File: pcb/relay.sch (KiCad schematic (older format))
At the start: 22 parts, among them IC1 ATTINY13-P, P1 CONN_01X02, P2 CONN_02X20, Q1 BC548, Q2 BC548, SW1 SW_PUSH, U1 78L05, U2 DX_MODULE

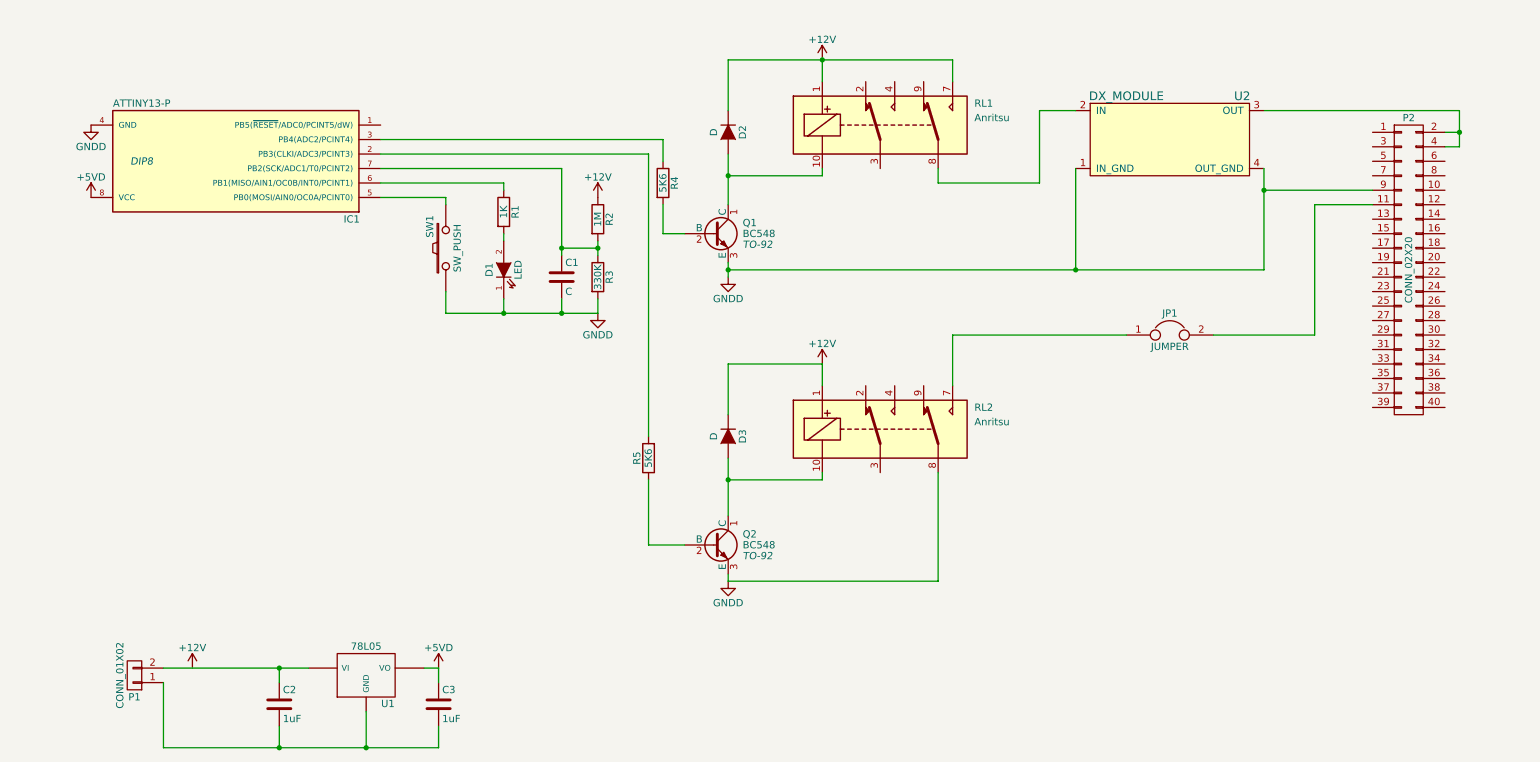
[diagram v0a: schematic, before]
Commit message: More work on PCB
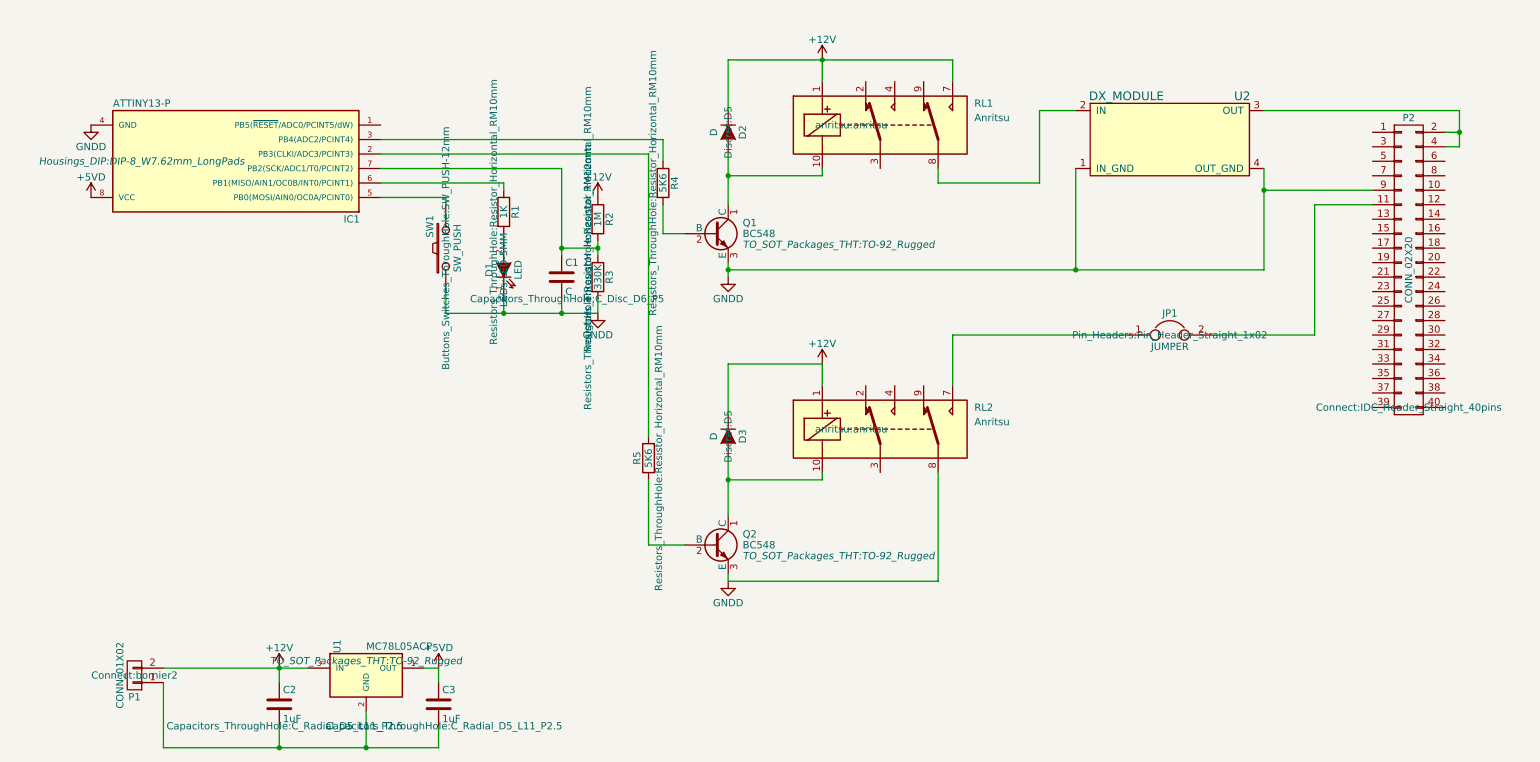
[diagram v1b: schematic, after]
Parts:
- removed U1: 78L05, symbol 78L05
- added U1: MC78L05ACP, TO_SOT_Packages_THT:TO-92_Rugged, symbol MC78L05ACP
- C1: footprint (none) -> Capacitors_ThroughHole:C_Disc_D6_P5
- C2, C3: footprint (none) -> Capacitors_ThroughHole:C_Radial_D5_L11_P2.5
- D1: footprint (none) -> LEDs:LED-5MM
- D2, D3: footprint (none) -> Discret:D5
- IC1: footprint DIP8 -> Housings_DIP:DIP-8_W7.62mm_LongPads
- JP1: footprint (none) -> Pin_Headers:Pin_Header_Straight_1x02
- P1: footprint (none) -> Connect:bornier2
- P2: footprint (none) -> Connect:IDC_Header_Straight_40pins
- Q1, Q2: footprint TO-92 -> TO_SOT_Packages_THT:TO-92_Rugged
- R1, R2, R3, R4, R5: footprint (none) -> Resistors_ThroughHole:Resistor_Horizontal_RM10mm
- RL1, RL2: footprint (none) -> anritsu:anritsu
- SW1: footprint (none) -> Buttons_Switches_ThroughHole:SW_PUSH-12mm
- U2: footprint (none) -> dx_module:dx_module
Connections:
- net +12V: now also C2.1, P1.2 (P2), U1.3 (IN)
- net +5VD: now also U1.1 (OUT)
- net at C2.2, C3.2, P1.1 (P1): now also U1.2 (GND)
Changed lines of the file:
@@
 LIBS:anritsu
 LIBS:dx_module
+LIBS:relay-cache
 EELAYER 25 0
 EELAYER END
@@
 F 0 "IC1" H 1150 1850 50  0000 C CNN
 F 1 "ATTINY13-P" H 2600 1050 50  0000 C CNN
-F 2 "DIP8" H 2600 1450 50  0000 C CIN
+F 2 "Housings_DIP:DIP-8_W7.62mm_LongPads" H 2600 1450 50  0000 C CIN
 F 3 "" H 1150 1800 50  0000 C CNN
 	1    1950 1450
@@
 F 0 "Q1" H 5450 2025 50  0000 L CNN
 F 1 "BC548" H 5450 1950 50  0000 L CNN
-F 2 "TO-92" H 5450 1875 50  0000 L CIN
+F 2 "TO_SOT_Packages_THT:TO-92_Rugged" H 5450 1875 50  0000 L CIN
 F 3 "" H 5250 1950 50  0000 L CNN
 	1    5250 1950
@@
 F 0 "Q2" H 5450 4175 50  0000 L CNN
 F 1 "BC548" H 5450 4100 50  0000 L CNN
-F 2 "TO-92" H 5450 4025 50  0000 L CIN
+F 2 "TO_SOT_Packages_THT:TO-92_Rugged" H 5450 4025 50  0000 L CIN
 F 3 "" H 5250 4100 50  0000 L CNN
 	1    5250 4100
@@
 $EndComp
 $Comp
-L GNDD #PWR?
+L GNDD #PWR01
 U 1 1 57CD5BEB
 P 5350 2250
-F 0 "#PWR?" H 5350 2000 50  0001 C CNN
+F 0 "#PWR01" H 5350 2000 50  0001 C CNN
 F 1 "GNDD" H 5350 2100 50  0000 C CNN
 F 2 "" H 5350 2250 50  0000 C CNN
@@
 $EndComp
 $Comp
-L GNDD #PWR?
+L GNDD #PWR02
 U 1 1 57CD5C09
 P 950 1200
-F 0 "#PWR?" H 950 950 50  0001 C CNN
+F 0 "#PWR02" H 950 950 50  0001 C CNN
 F 1 "GNDD" H 950 1050 50  0000 C CNN
 F 2 "" H 950 1200 50  0000 C CNN
@@
 $EndComp
 $Comp
-L +5VD #PWR?
+L +5VD #PWR03
 U 1 1 57CD5C27
 P 950 1700
-F 0 "#PWR?" H 950 1550 50  0001 C CNN
+F 0 "#PWR03" H 950 1550 50  0001 C CNN
 F 1 "+5VD" H 950 1840 50  0000 C CNN
 F 2 "" H 950 1700 50  0000 C CNN
@@
 F 0 "D2" H 5350 1350 50  0000 C CNN
 F 1 "D" H 5350 1150 50  0000 C CNN
-F 2 "" H 5350 1250 50  0000 C CNN
+F 2 "Discret:D5" H 5350 1250 50  0000 C CNN
 F 3 "" H 5350 1250 50  0000 C CNN
 	1    5350 1250
@@
 F 0 "D3" H 5350 3450 50  0000 C CNN
 F 1 "D" H 5350 3250 50  0000 C CNN
-F 2 "" H 5350 3350 50  0000 C CNN
+F 2 "Discret:D5" H 5350 3350 50  0000 C CNN
 F 3 "" H 5350 3350 50  0000 C CNN
 	1    5350 3350
@@
 F 0 "R4" V 4980 1600 50  0000 C CNN
 F 1 "5K6" V 4900 1600 50  0000 C CNN
-F 2 "" V 4830 1600 50  0000 C CNN
+F 2 "Resistors_ThroughHole:Resistor_Horizontal_RM10mm" V 4830 1600 50  0000 C CNN
 F 3 "" H 4900 1600 50  0000 C CNN
 	1    4900 1600
@@
 F 0 "R5" V 4880 3500 50  0000 C CNN
 F 1 "5K6" V 4800 3500 50  0000 C CNN
-F 2 "" V 4730 3500 50  0000 C CNN
+F 2 "Resistors_ThroughHole:Resistor_Horizontal_RM10mm" V 4730 3500 50  0000 C CNN
 F 3 "" H 4800 3500 50  0000 C CNN
 	1    4800 3500
@@
 F 0 "R2" V 4530 1850 50  0000 C CNN
 F 1 "1M" V 4450 1850 50  0000 C CNN
-F 2 "" V 4380 1850 50  0000 C CNN
+F 2 "Resistors_ThroughHole:Resistor_Horizontal_RM10mm" V 4380 1850 50  0000 C CNN
 F 3 "" H 4450 1850 50  0000 C CNN
 	1    4450 1850
@@
 F 0 "R3" V 4530 2250 50  0000 C CNN
 F 1 "330K" V 4450 2250 50  0000 C CNN
-F 2 "" V 4380 2250 50  0000 C CNN
+F 2 "Resistors_ThroughHole:Resistor_Horizontal_RM10mm" V 4380 2250 50  0000 C CNN
 F 3 "" H 4450 2250 50  0000 C CNN
 	1    4450 2250
@@
 $EndComp
 $Comp
-L +12V #PWR?
+L +12V #PWR04
 U 1 1 57CD66EF
 P 4450 1700
-F 0 "#PWR?" H 4450 1550 50  0001 C CNN
+F 0 "#PWR04" H 4450 1550 50  0001 C CNN
 F 1 "+12V" H 4450 1840 50  0000 C CNN
 F 2 "" H 4450 1700 50  0000 C CNN
@@
 F 0 "C1" H 4225 2350 50  0000 L CNN
 F 1 "C" H 4225 2150 50  0000 L CNN
-F 2 "" H 4238 2100 50  0000 C CNN
+F 2 "Capacitors_ThroughHole:C_Disc_D6_P5" H 4238 2100 50  0000 C CNN
 F 3 "" H 4200 2250 50  0000 C CNN
 	1    4200 2250
@@
 $EndComp
 $Comp
-L GNDD #PWR?
+L GNDD #PWR05
 U 1 1 57CD68E3
 P 4450 2500
-F 0 "#PWR?" H 4450 2250 50  0001 C CNN
+F 0 "#PWR05" H 4450 2250 50  0001 C CNN
 F 1 "GNDD" H 4450 2350 50  0000 C CNN
 F 2 "" H 4450 2500 50  0000 C CNN
@@
 F 0 "P1" H 1250 5150 50  0000 C CNN
 F 1 "CONN_01X02" V 1350 5000 50  0000 C CNN
-F 2 "" H 1250 5000 50  0000 C CNN
+F 2 "Connect:bornier2" H 1250 5000 50  0000 C CNN
 F 3 "" H 1250 5000 50  0000 C CNN
 	1    1250 5000
@@
 F 0 "C2" H 2275 5300 50  0000 L CNN
 F 1 "1uF" H 2275 5100 50  0000 L CNN
-F 2 "" H 2288 5050 50  0000 C CNN
+F 2 "Capacitors_ThroughHole:C_Radial_D5_L11_P2.5" H 2288 5050 50  0000 C CNN
 F 3 "" H 2250 5200 50  0000 C CNN
 	1    2250 5200
@@
 F 0 "C3" H 3375 5300 50  0000 L CNN
 F 1 "1uF" H 3375 5100 50  0000 L CNN
-F 2 "" H 3388 5050 50  0000 C CNN
+F 2 "Capacitors_ThroughHole:C_Radial_D5_L11_P2.5" H 3388 5050 50  0000 C CNN
 F 3 "" H 3350 5200 50  0000 C CNN
 	1    3350 5200
@@
 $EndComp
 $Comp
-L 78L05 U1
-U 1 1 57CD72E7
-P 2850 5000
-F 0 "U1" H 3000 4804 50  0000 C CNN
-F 1 "78L05" H 2850 5200 50  0000 C CNN
-F 2 "" H 2850 5000 50  0000 C CNN
-F 3 "" H 2850 5000 50  0000 C CNN
-	1    2850 5000
-	1    0    0    -1
-$EndComp
-$Comp
-L +5VD #PWR?
+L +5VD #PWR06
 U 1 1 57CD74DA
 P 3350 4950
-F 0 "#PWR?" H 3350 4800 50  0001 C CNN
+F 0 "#PWR06" H 3350 4800 50  0001 C CNN
 F 1 "+5VD" H 3350 5090 50  0000 C CNN
 F 2 "" H 3350 4950 50  0000 C CNN
@@
 $EndComp
 $Comp
-L +12V #PWR?
+L +12V #PWR07
 U 1 1 57CD7D1E
-P 1650 4950
-F 0 "#PWR?" H 1650 4800 50  0001 C CNN
-F 1 "+12V" H 1650 5090 50  0000 C CNN
-F 2 "" H 1650 4950 50  0000 C CNN
-F 3 "" H 1650 4950 50  0000 C CNN
-	1    1650 4950
+P 2250 4950
+F 0 "#PWR07" H 2250 4800 50  0001 C CNN
+F 1 "+12V" H 2250 5090 50  0000 C CNN
+F 2 "" H 2250 4950 50  0000 C CNN
+F 3 "" H 2250 4950 50  0000 C CNN
+	1    2250 4950
 	1    0    0    -1
 $EndComp
@@
 F 0 "R1" V 3880 1800 50  0000 C CNN
 F 1 "1K" V 3800 1800 50  0000 C CNN
-F 2 "" V 3730 1800 50  0000 C CNN
+F 2 "Resistors_ThroughHole:Resistor_Horizontal_RM10mm" V 3730 1800 50  0000 C CNN
 F 3 "" H 3800 1800 50  0000 C CNN
 	1    3800 1800
@@
 F 0 "D1" H 3800 2300 50  0000 C CNN
 F 1 "LED" H 3800 2100 50  0000 C CNN
-F 2 "" H 3800 2200 50  0000 C CNN
+F 2 "LEDs:LED-5MM" H 3800 2200 50  0000 C CNN
 F 3 "" H 3800 2200 50  0000 C CNN
 	1    3800 2200
@@
 F 0 "SW1" H 3550 2160 50  0000 C CNN
 F 1 "SW_PUSH" H 3400 1970 50  0000 C CNN
-F 2 "" H 3400 2050 50  0000 C CNN
+F 2 "Buttons_Switches_ThroughHole:SW_PUSH-12mm" H 3400 2050 50  0000 C CNN
 F 3 "" H 3400 2050 50  0000 C CNN
 	1    3400 2050
@@
 F 0 "P2" H 10050 3250 50  0000 C CNN
 F 1 "CONN_02X20" V 10050 2200 50  0000 C CNN
-F 2 "" H 10050 1250 50  0000 C CNN
+F 2 "Connect:IDC_Header_Straight_40pins" H 10050 1250 50  0000 C CNN
 F 3 "" H 10050 1250 50  0000 C CNN
 	1    10050 2200
@@
 $EndComp
 $Comp
-L +12V #PWR?
+L +12V #PWR08
 U 1 1 57CD90B3
 P 6000 2850
-F 0 "#PWR?" H 6000 2700 50  0001 C CNN
+F 0 "#PWR08" H 6000 2700 50  0001 C CNN
 F 1 "+12V" H 6000 2990 50  0000 C CNN
 F 2 "" H 6000 2850 50  0000 C CNN
@@
 $EndComp
 $Comp
-L +12V #PWR?
+L +12V #PWR09
 U 1 1 57CD90EF
 P 6000 750
-F 0 "#PWR?" H 6000 600 50  0001 C CNN
+F 0 "#PWR09" H 6000 600 50  0001 C CNN
 F 1 "+12V" H 6000 890 50  0000 C CNN
 F 2 "" H 6000 750 50  0000 C CNN
@@
 $EndComp
 $Comp
-L GNDD #PWR?
+L GNDD #PWR010
 U 1 1 57CD9222
 P 5350 4350
-F 0 "#PWR?" H 5350 4100 50  0001 C CNN
+F 0 "#PWR010" H 5350 4100 50  0001 C CNN
 F 1 "GNDD" H 5350 4200 50  0000 C CNN
 F 2 "" H 5350 4350 50  0000 C CNN
@@
 F 0 "RL1" H 7050 1350 50  0000 L CNN
 F 1 "Anritsu" H 7050 1250 50  0000 L CNN
-F 2 "" H 6200 1200 50  0000 C CNN
+F 2 "anritsu:anritsu" H 6200 1200 50  0000 C CNN
 F 3 "" H 6200 1200 50  0000 C CNN
 	1    6200 1200
@@
 F 0 "RL2" H 7050 3450 50  0000 L CNN
 F 1 "Anritsu" H 7050 3350 50  0000 L CNN
-F 2 "" H 6200 3300 50  0000 C CNN
+F 2 "anritsu:anritsu" H 6200 3300 50  0000 C CNN
 F 3 "" H 6200 3300 50  0000 C CNN
 	1    6200 3300
@@
 F 0 "U2" H 8900 1900 60  0000 C CNN
 F 1 "DX_MODULE" H 8100 1900 60  0000 C CNN
-F 2 "" H 8400 1450 60  0001 C CNN
+F 2 "dx_module:dx_module" H 8400 1450 60  0001 C CNN
 F 3 "" H 8400 1450 60  0001 C CNN
 	1    8400 1450
@@
 F 0 "JP1" H 8400 2800 50  0000 C CNN
 F 1 "JUMPER" H 8400 2570 50  0000 C CNN
-F 2 "" H 8400 2650 50  0000 C CNN
+F 2 "Pin_Headers:Pin_Header_Straight_1x02" H 8400 2650 50  0000 C CNN
 F 3 "" H 8400 2650 50  0000 C CNN
 	1    8400 2650
@@
 Wire Wire Line
 	9400 1750 9800 1750
+$Comp
+L MC78L05ACP U1
+U 1 1 57D0150E
+P 2850 5000
+F 0 "U1" V 2650 5200 50  0000 C CNN
+F 1 "MC78L05ACP" H 2850 5200 50  0000 L CNN
+F 2 "TO_SOT_Packages_THT:TO-92_Rugged" H 2850 5100 50  0000 C CIN
+F 3 "" H 2850 5000 50  0000 C CNN
+	1    2850 5000
+	1    0    0    -1
+$EndComp
 $EndSCHEMATC
